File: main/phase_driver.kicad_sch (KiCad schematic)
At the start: 10 parts, among them Q1001 TK4R3E06PL, Q1002 TK4R3E06PL, U1001 LM2105

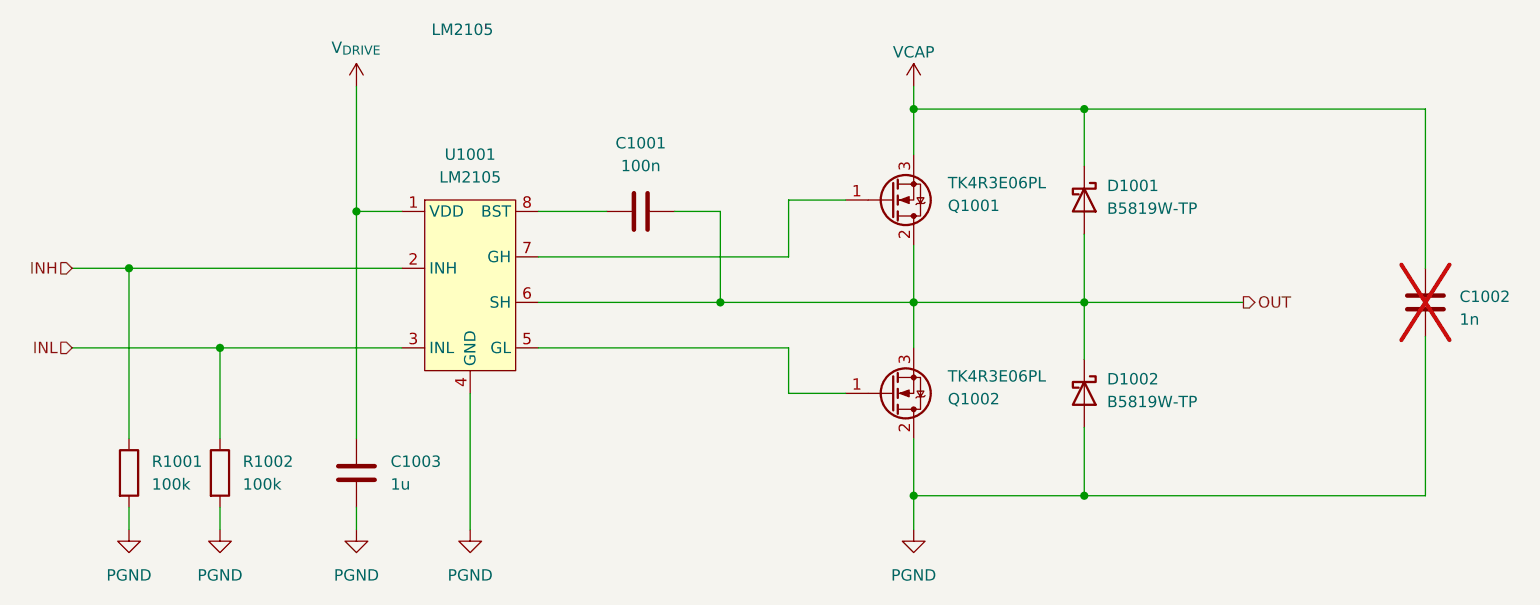
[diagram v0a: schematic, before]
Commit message: Sent to fab
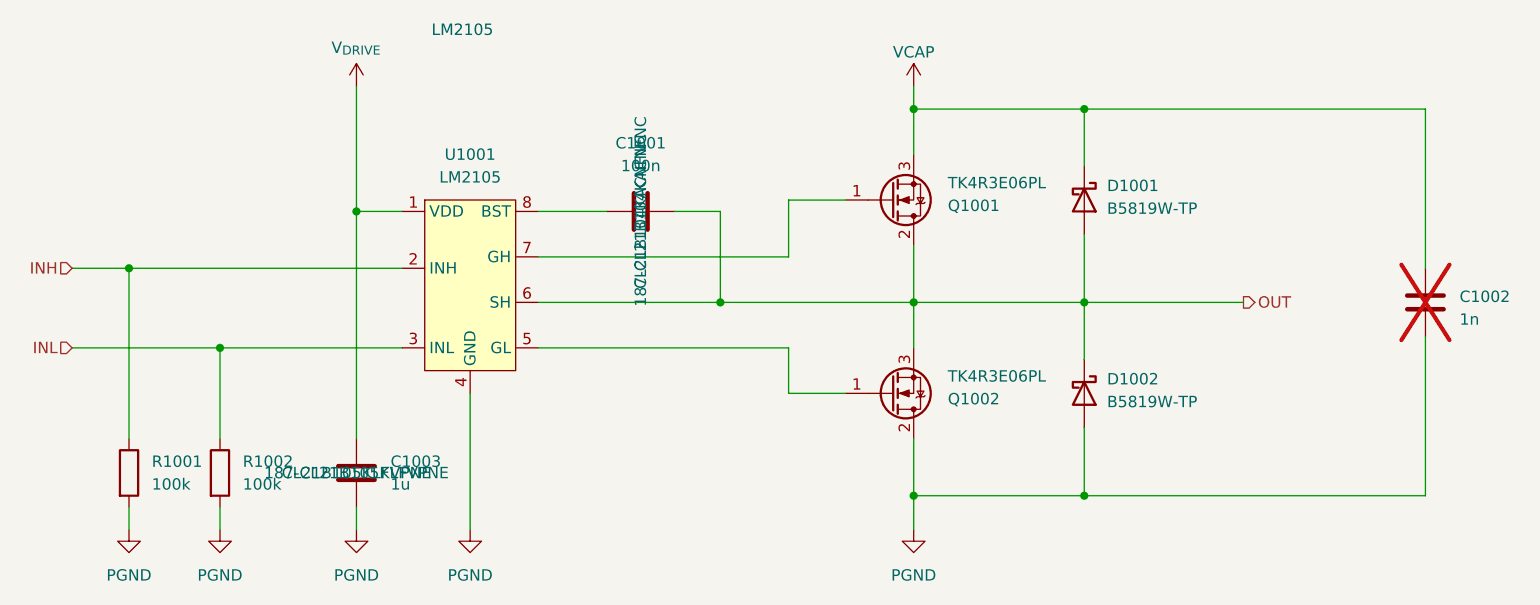
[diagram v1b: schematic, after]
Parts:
- C1001: MPN (none) -> CL21B104KACNFNC; Mouser SKU (none) -> 187-CL21B104KACNFNC
- C1003: MPN (none) -> CL21B105KLFVPNE; Mouser SKU (none) -> 187-CL21B105KLFVPNE
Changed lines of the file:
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@@
+			)
+		)
+		(property "Quantity" ""
+			(at 190.5 57.15 0)
+			(effects
+				(font
+					(size 1.27 1.27)
+				)
 			)
 		)
@@
 			)
 		)
+		(property "MPN" "CL21B104KACNFNC "
+			(at 140.97 58.42 0)
+			(effects
+				(font
+					(size 1.27 1.27)
+				)
+			)
+		)
+		(property "Mouser SKU" " 187-CL21B104KACNFNC "
+			(at 140.97 58.42 0)
+			(effects
+				(font
+					(size 1.27 1.27)
+				)
+			)
+		)
+		(property "Quantity" ""
+			(at 140.97 58.42 0)
+			(effects
+				(font
+					(size 1.27 1.27)
+				)
+			)
+		)
 		(pin "1"
 		)
@@
 			)
 		)
+		(property "Quantity" ""
+			(at 228.6 68.58 0)
+			(effects
+				(font
+					(size 1.27 1.27)
+				)
+			)
+		)
 		(pin "1"
 		)
@@
 			)
 		)
+		(property "Quantity" ""
+			(at 83.82 87.63 0)
+			(effects
+				(font
+					(size 1.27 1.27)
+				)
+			)
+		)
 		(pin "1"
 		)
@@
 			)
 		)
+		(property "Quantity" ""
+			(at 121.92 66.04 0)
+			(effects
+				(font
+					(size 1.27 1.27)
+				)
+			)
+		)
 		(pin "3"
 		)
@@
 			)
 		)
+		(property "Quantity" ""
+			(at 168.91 78.74 0)
+			(effects
+				(font
+					(size 1.27 1.27)
+				)
+			)
+		)
 		(pin "1"
 		)
@@
 			)
 		)
+		(property "Quantity" ""
+			(at 93.98 87.63 0)
+			(effects
+				(font
+					(size 1.27 1.27)
+				)
+			)
+		)
 		(pin "1"
 		)
@@
 			)
 		)
+		(property "Quantity" ""
+			(at 190.5 78.74 0)
+			(effects
+				(font
+					(size 1.27 1.27)
+				)
+			)
+		)
 		(pin "2"
 		)
@@
 			)
 		)
+		(property "Quantity" ""
+			(at 168.91 57.15 0)
+			(effects
+				(font
+					(size 1.27 1.27)
+				)
+			)
+		)
 		(pin "1"
 		)
@@
 			)
 		)
+		(property "MPN" "CL21B105KLFVPNE "
+			(at 109.22 87.63 0)
+			(effects
+				(font
+					(size 1.27 1.27)
+				)
+			)
+		)
+		(property "Mouser SKU" " 187-CL21B105KLFVPNE "
+			(at 109.22 87.63 0)
+			(effects
+				(font
+					(size 1.27 1.27)
+				)
+			)
+		)
+		(property "Quantity" ""
+			(at 109.22 87.63 0)
+			(effects
+				(font
+					(size 1.27 1.27)
+				)
+			)
+		)
